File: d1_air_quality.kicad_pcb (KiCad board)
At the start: 2 copper layers, 27.4 x 42.7 mm, 10 parts, among them J1 GP2Y10, J2 I2C1, J3 I2C2, J4 I2C3, J5 Conn_01x07_Male, U1 WeMos_mini

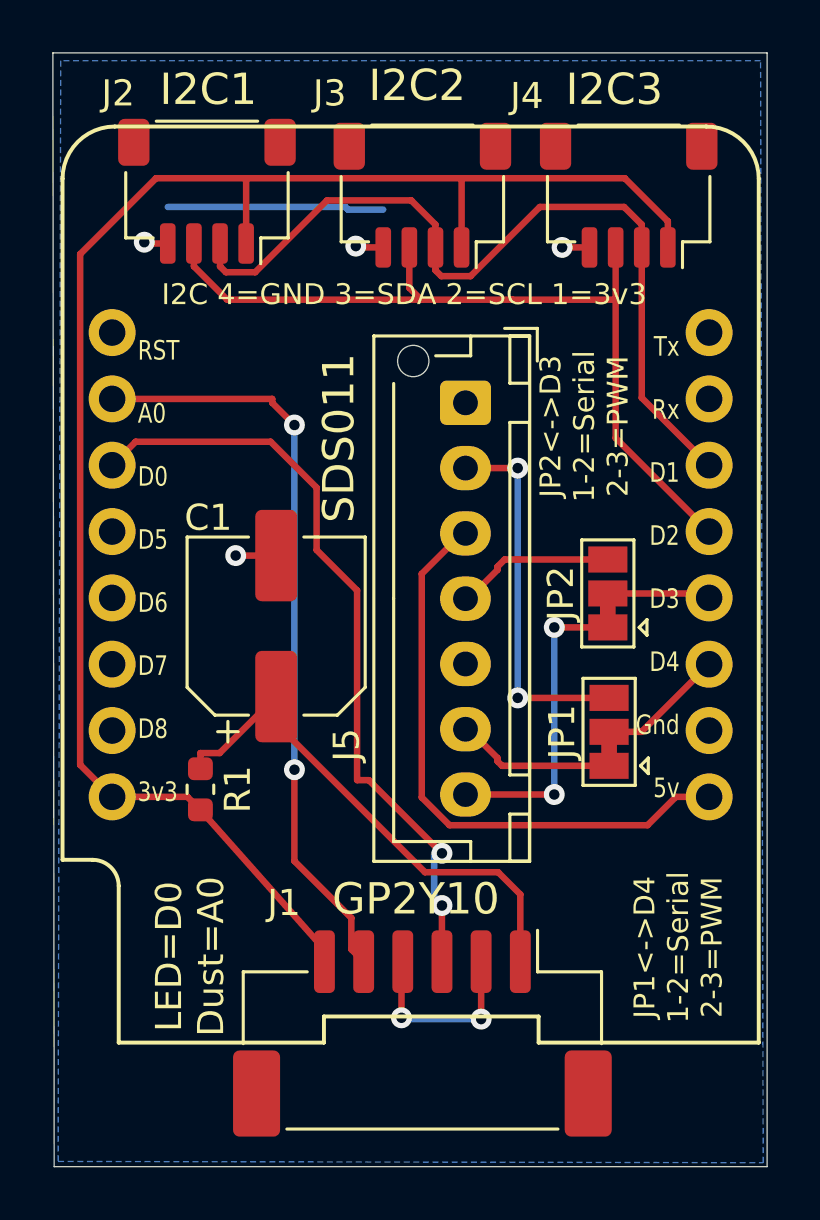
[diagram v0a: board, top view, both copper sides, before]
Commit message: Add basic doco
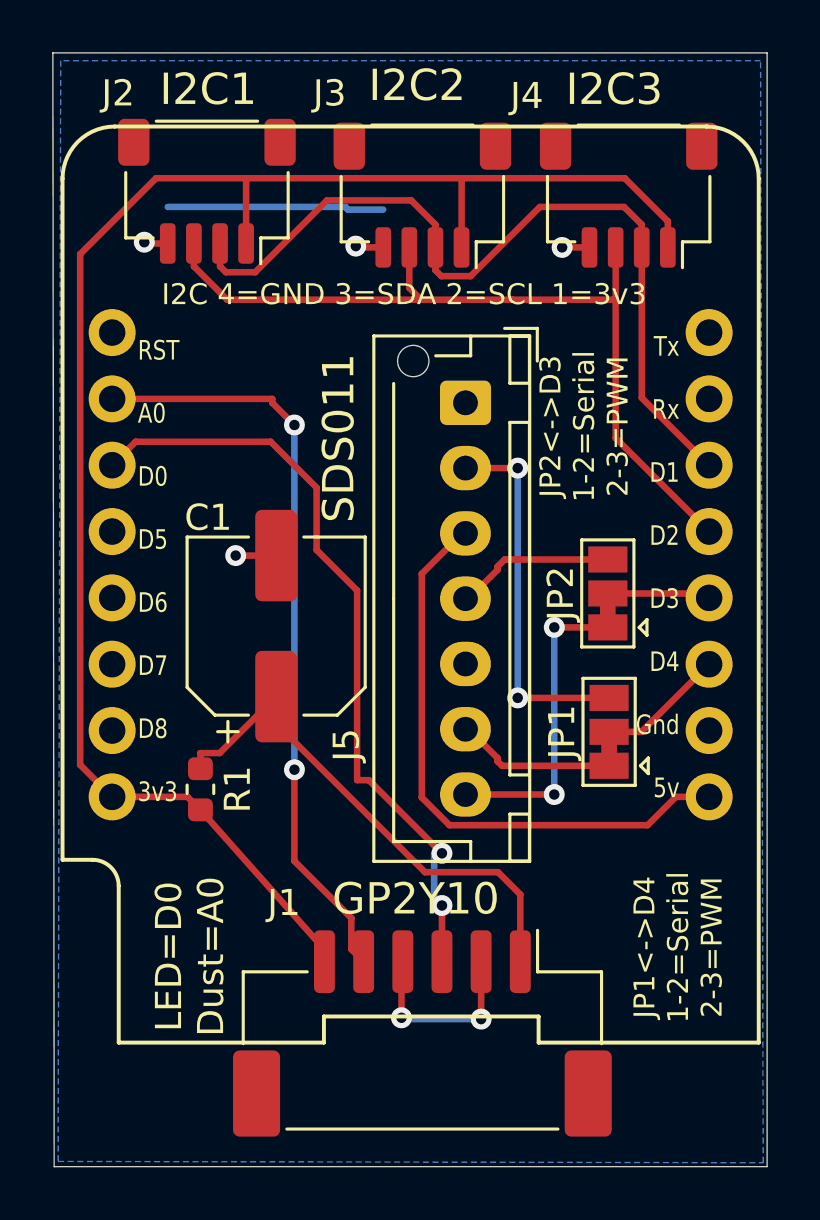
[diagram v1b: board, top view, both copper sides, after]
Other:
- net class Default removed
